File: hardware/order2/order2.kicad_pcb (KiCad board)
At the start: 2 copper layers, 137 x 65 mm, 99 parts, among them IC1 ATMEGA88A-A, J1 RJ45_8P8C_8FACH, K1 pow_sel, P1 UART, P2 Shield, P3 i2c_pow, P4 i2c_chain, P5 12Vin, P6 HOHLBUCHSE, P7 Vccin, P8 ISP, P9 5Vin, SW1 SW1, SW2 SCHALTER_2POL, SW3 SW_RESET, U1 LM7805, U2 ST485, U3 ST485, U4 ST485, U5 ST485, U6 ST485, U7 ST485, U8 ST485, U9 ST485, X1 20MHz, m3_loch VAL**

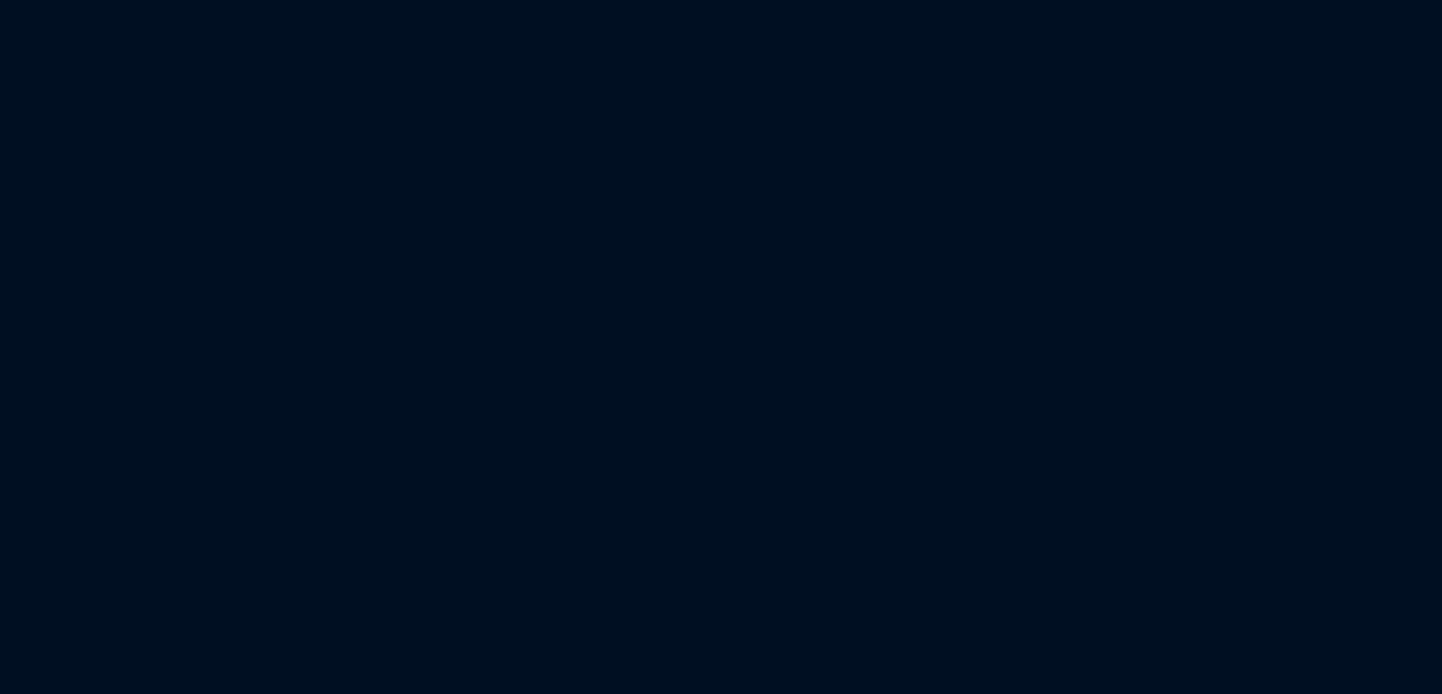
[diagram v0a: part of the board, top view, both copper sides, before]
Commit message: order2_s2
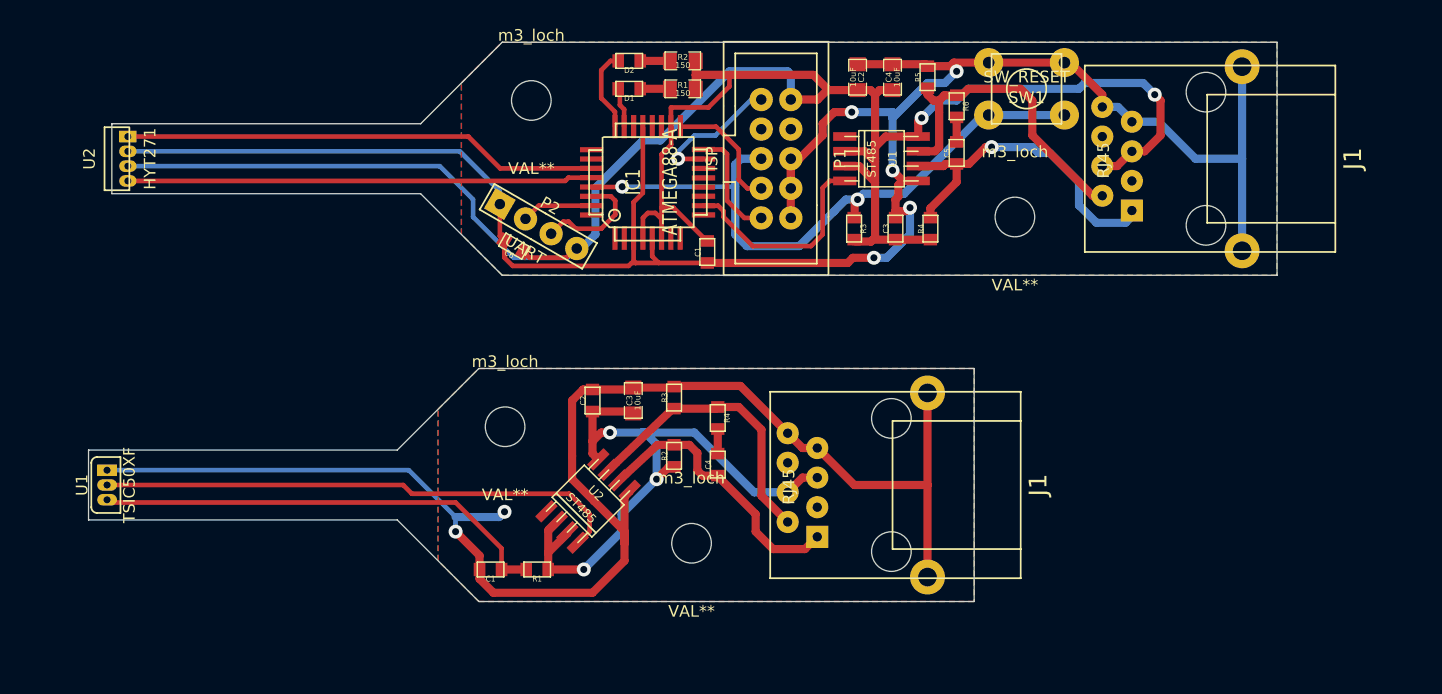
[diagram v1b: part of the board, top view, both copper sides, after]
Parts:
- added C1: 100nF, SM0603_big, F.Cu at (79.1, 44.0)
- added C1: 100nF, SM0603_big, F.Cu at (60.5, 71.2)
- added C2: 10uF, SM0805_big, F.Cu at (92.0, 29.0)
- added C2: 100nF, SM0603_big, F.Cu at (69.2, 56.8)
- added C3: 100nF, SM0603_big, F.Cu at (95.2, 42.0)
- added C3: 10uF, SM0805_big, F.Cu at (72.8, 56.8)
- added C4: 10uF, SM0805_big, F.Cu at (95.0, 29.0)
- added C4: 100nF, SM0603_big, F.Cu at (80.0, 62.2)
- added C5: 100nF, SM0603_big, F.Cu at (100.5, 35.5)
- added C6: 100nF, SM0603_big, F.Cu at (62.5, 43.5)
- added D1: LED, SM0603_big, F.Cu at (72.4, 30.0)
- added D2: LED, SM0603_big, F.Cu at (72.4, 27.6)
- added IC1: ATMEGA88-A, TQFP32, F.Cu at (74.0, 38.0)
- added J1: RJ45, RJ45_8P8_simple, F.Cu at (113.0, 36.0)
- added J1: RJ45, RJ45_8P8_simple, F.Cu at (86.0, 64.0)
- added P1: ISP, wannenstecker_2x5_rm254, F.Cu at (85.0, 36.0)
- added P2: UART, Stiftleiste_4x1, F.Cu at (64.6, 41.8)
- added R1: 150, SM0805_big, F.Cu at (77.0, 30.0)
- added R1: 220, SM0603_big, F.Cu at (64.5, 71.2)
- added R2: 150, SM0805_big, F.Cu at (77.0, 27.6)
- added R2: 22k, SM0603_big, F.Cu at (76.2, 61.5)
- added R3: 10k, SM0603_big, F.Cu at (91.7, 42.0)
- added R3: 22k, SM0603_big, F.Cu at (76.2, 56.5)
- added R4: 22k, SM0603_big, F.Cu at (98.2, 42.0)
- added R4: 120, SM0603_big, F.Cu at (80.0, 58.2)
- added R5: 22k, SM0603_big, F.Cu at (98.0, 29.0)
- added R6: 120, SM0603_big, F.Cu at (100.5, 31.5)
- added SW1: SW_RESET, Taster_6mm, F.Cu at (106.5, 30.0)
- added U1: ST485, st485, F.Cu at (96.0, 36.0)
- added U1: TSIC50XF, Tsic_TO92, F.Cu at (29.5, 64.0)
- added U2: HYT271, HYT271, F.Cu at (29.5, 36.0)
- added U2: ST485, st485, F.Cu at (70.2, 64.0)
- added m3_loch: VAL**, m3_loch, F.Cu at (105.5, 41.0)
- added m3_loch: VAL**, m3_loch, F.Cu at (64.0, 31.0)
- added m3_loch: VAL**, m3_loch, F.Cu at (77.8, 69.0)
- added m3_loch: VAL**, m3_loch, F.Cu at (61.8, 59.0)
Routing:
- net GND: track 883.2 -> 1194.5 mm, vias 3 -> 10
- net VCC: track 556.5 -> 806.0 mm, vias 3 -> 8
- net /RESET: track 106.9 -> 162.7 mm, vias 2 -> 4
- net /za: track 0.00 -> 53.3 mm, vias 0 -> 1
- net /zb: track 0.00 -> 52.6 mm
- net N-000007: track 3.76 -> 49.3 mm
- net /SDA: track 81.2 -> 122.1 mm
- net /SCL: track 89.2 -> 129.1 mm
- net N-0000010: track 0.00 -> 39.5 mm
- net /DI: track 0.00 -> 18.5 mm
- net /MOSI: track 49.6 -> 61.4 mm, vias 2 -> 3
- net /SCK: track 11.9 -> 22.5 mm
- net /RX: track 46.4 -> 56.4 mm
- net /MISO: track 8.73 -> 18.5 mm
- net /LED2: track 17.8 -> 24.9 mm
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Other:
- board size 137 x 65 mm -> 137 x 159 mm
- rule trace_min: 0.4 -> 0.254
